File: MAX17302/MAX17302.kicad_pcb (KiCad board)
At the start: 4 copper layers, 17.9 x 47 mm, 13 parts, among them J1 Conn_01x02, J2 Conn_01x02, J3 Conn_01x03, Q1 Q_NMOS_DSG, Q2 Q_NMOS_DSG, U1 MAX17302G+T

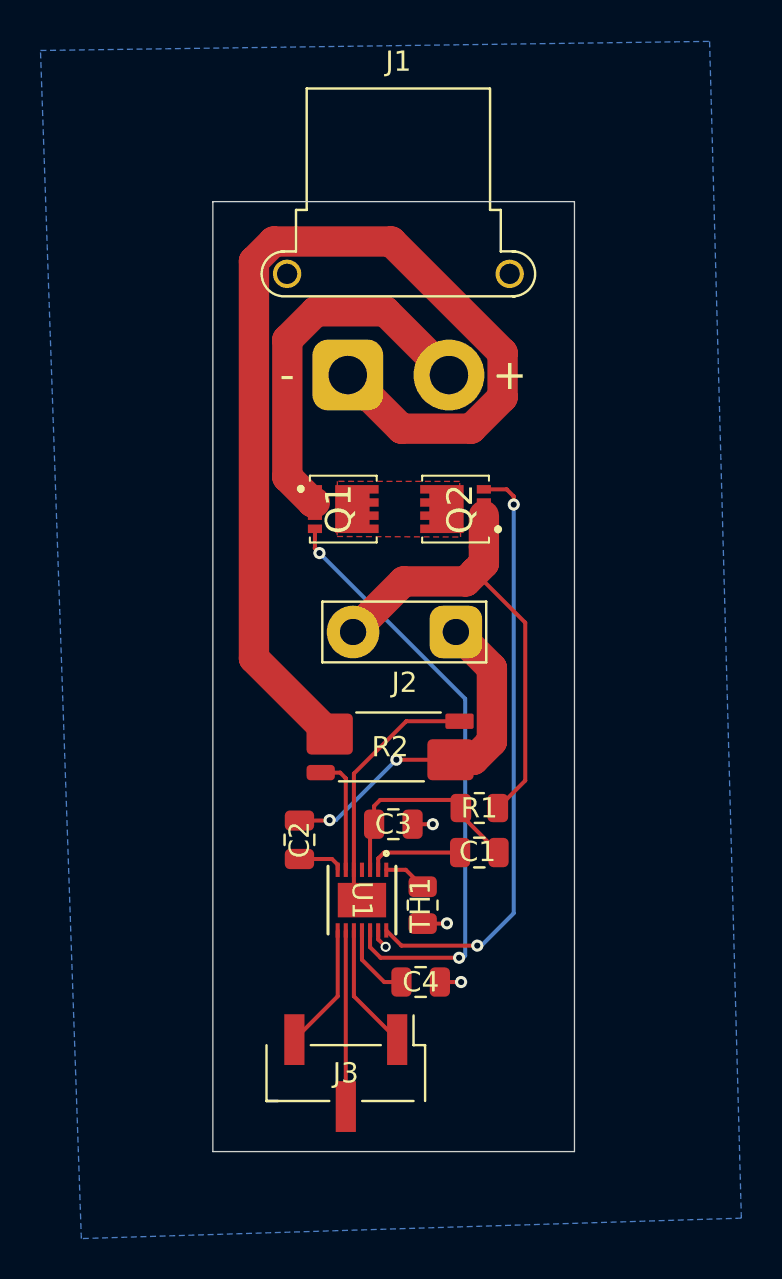
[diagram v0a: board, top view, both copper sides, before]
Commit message: Add files via upload
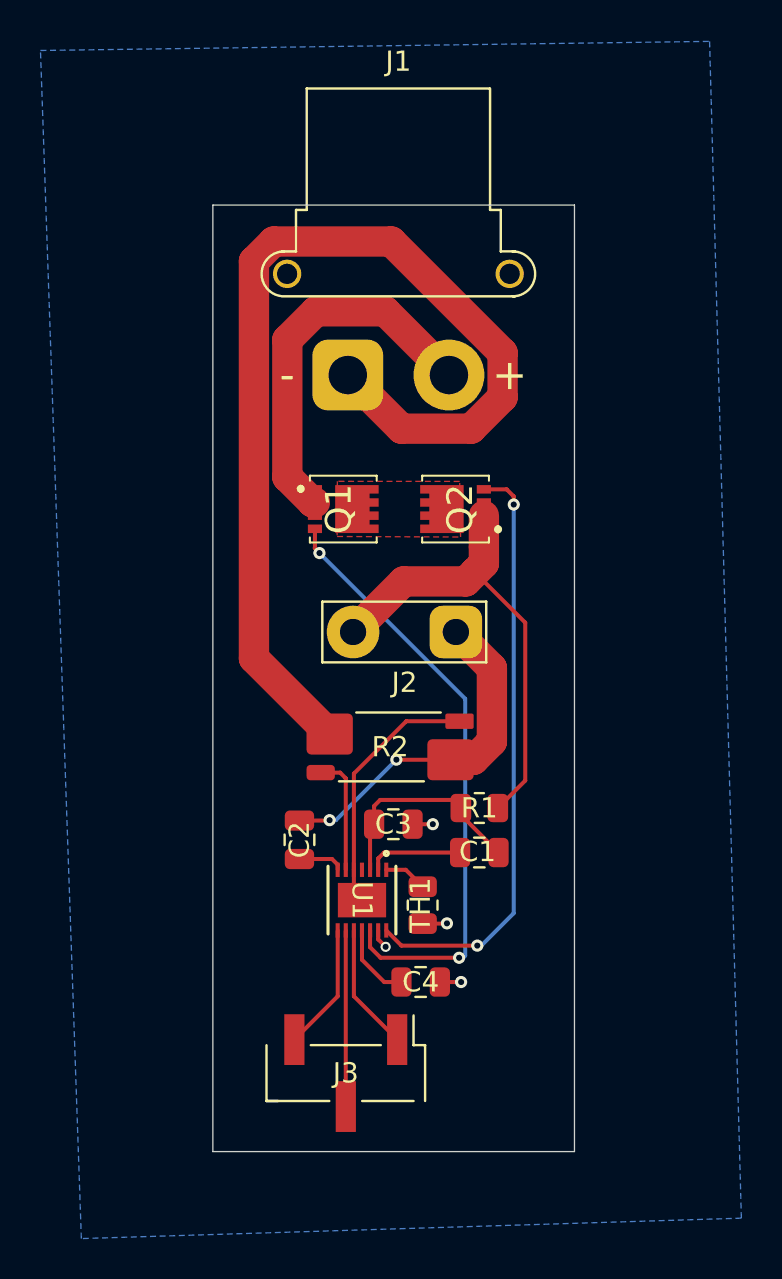
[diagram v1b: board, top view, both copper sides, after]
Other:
- board size 17.9 x 47 mm -> 17.9 x 46.8 mm
